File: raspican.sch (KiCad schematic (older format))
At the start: 3 parts, among them P1 CONN_13X2

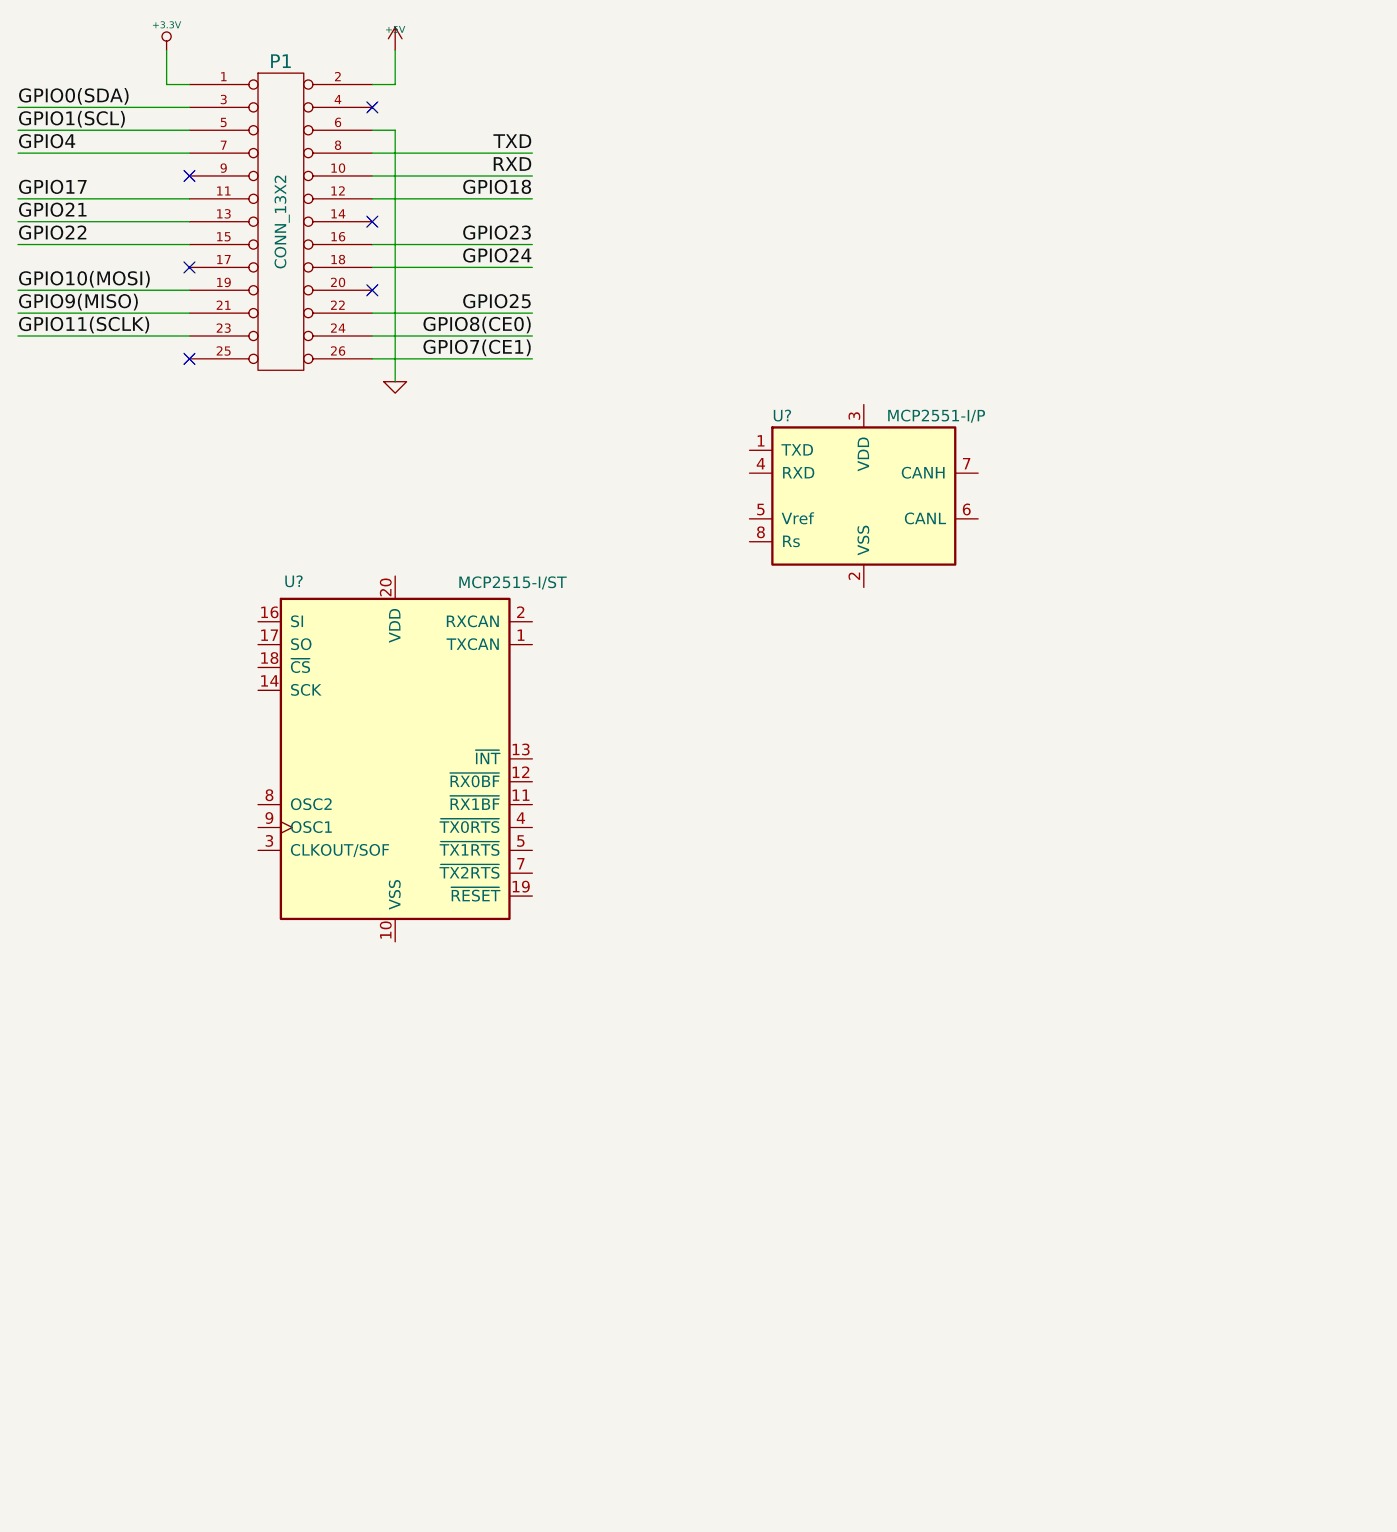
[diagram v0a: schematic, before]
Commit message: start wiring stuff up
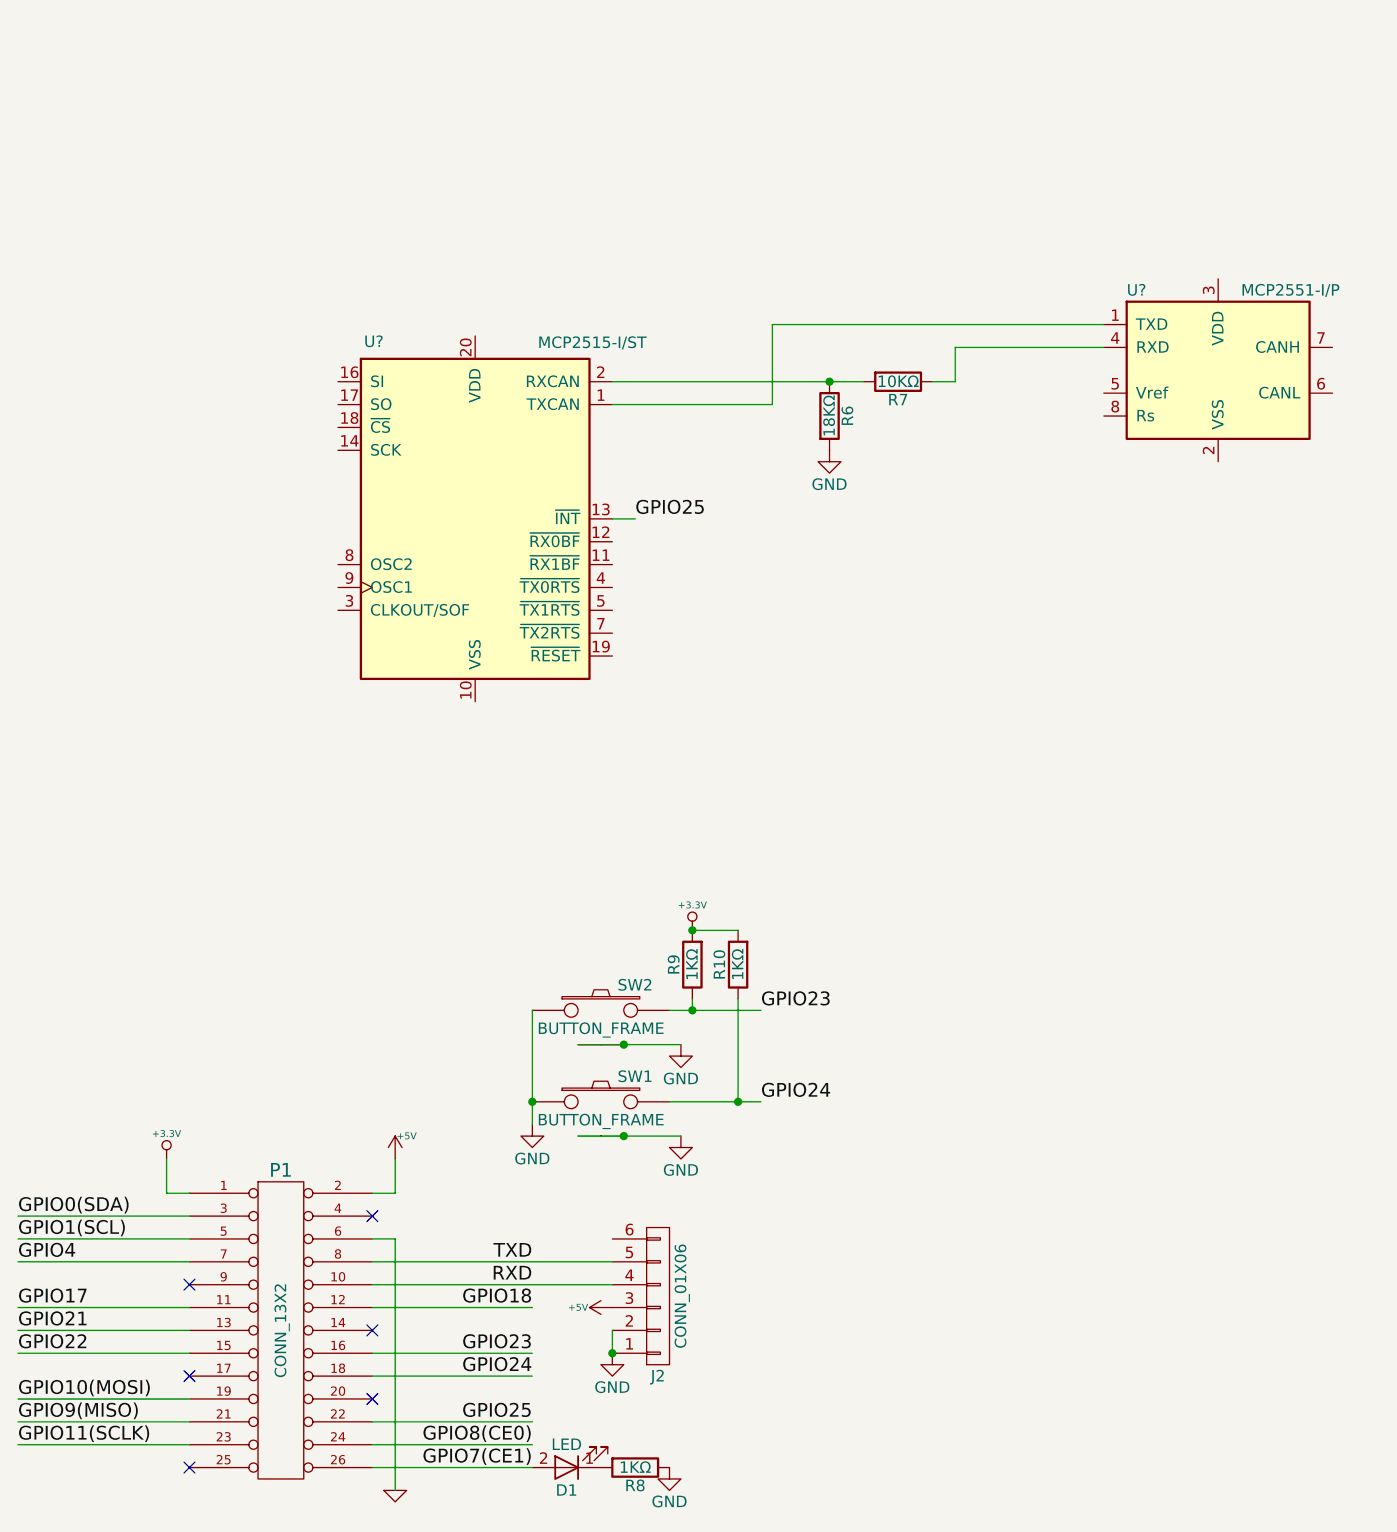
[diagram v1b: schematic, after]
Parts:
- added D1: LED, symbol LED
- added J2: CONN_01X06, symbol CONN_01X06
- added R10, R8, R9: 1KΩ, symbol R
- added R6: 18KΩ, symbol R
- added R7: 10KΩ, symbol R
- added SW1, SW2: BUTTON_FRAME, symbol BUTTON_FRAME
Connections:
- net +3.3V: now also R10.2, R9.2
- net +5V: now also J2.3 (P3)
- net GND: now also J2.1 (P1), J2.2 (P2), R6.2, R8.1, SW1.1, SW1.4, SW1.5, SW2.1, SW2.4, SW2.5
- net GPIO23: now also R9.1, SW2.2
- net GPIO24: now also R10.1, SW1.2
- net GPIO25: now also U?.13 (~INT)
- net GPIO7(CE1): now also D1.2 (A)
- net RXD: now also J2.4 (P4)
- net TXD: now also J2.5 (P5)
- net at U?.1 (TXCAN): now also U?.1 (TXD)
- net at U?.2 (RXCAN): now also R6.1, R7.2
- net at U?.4 (RXD): now also R7.1
- new net: D1.1 (K), R8.2
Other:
- moved on the sheet: P1, U?
